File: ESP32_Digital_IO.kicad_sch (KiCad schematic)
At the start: 23 parts, among them J2 217179-0001, J3 DIGITAL_IO_3V3, U3 ESP32-S3-WROOM-1-N16R8

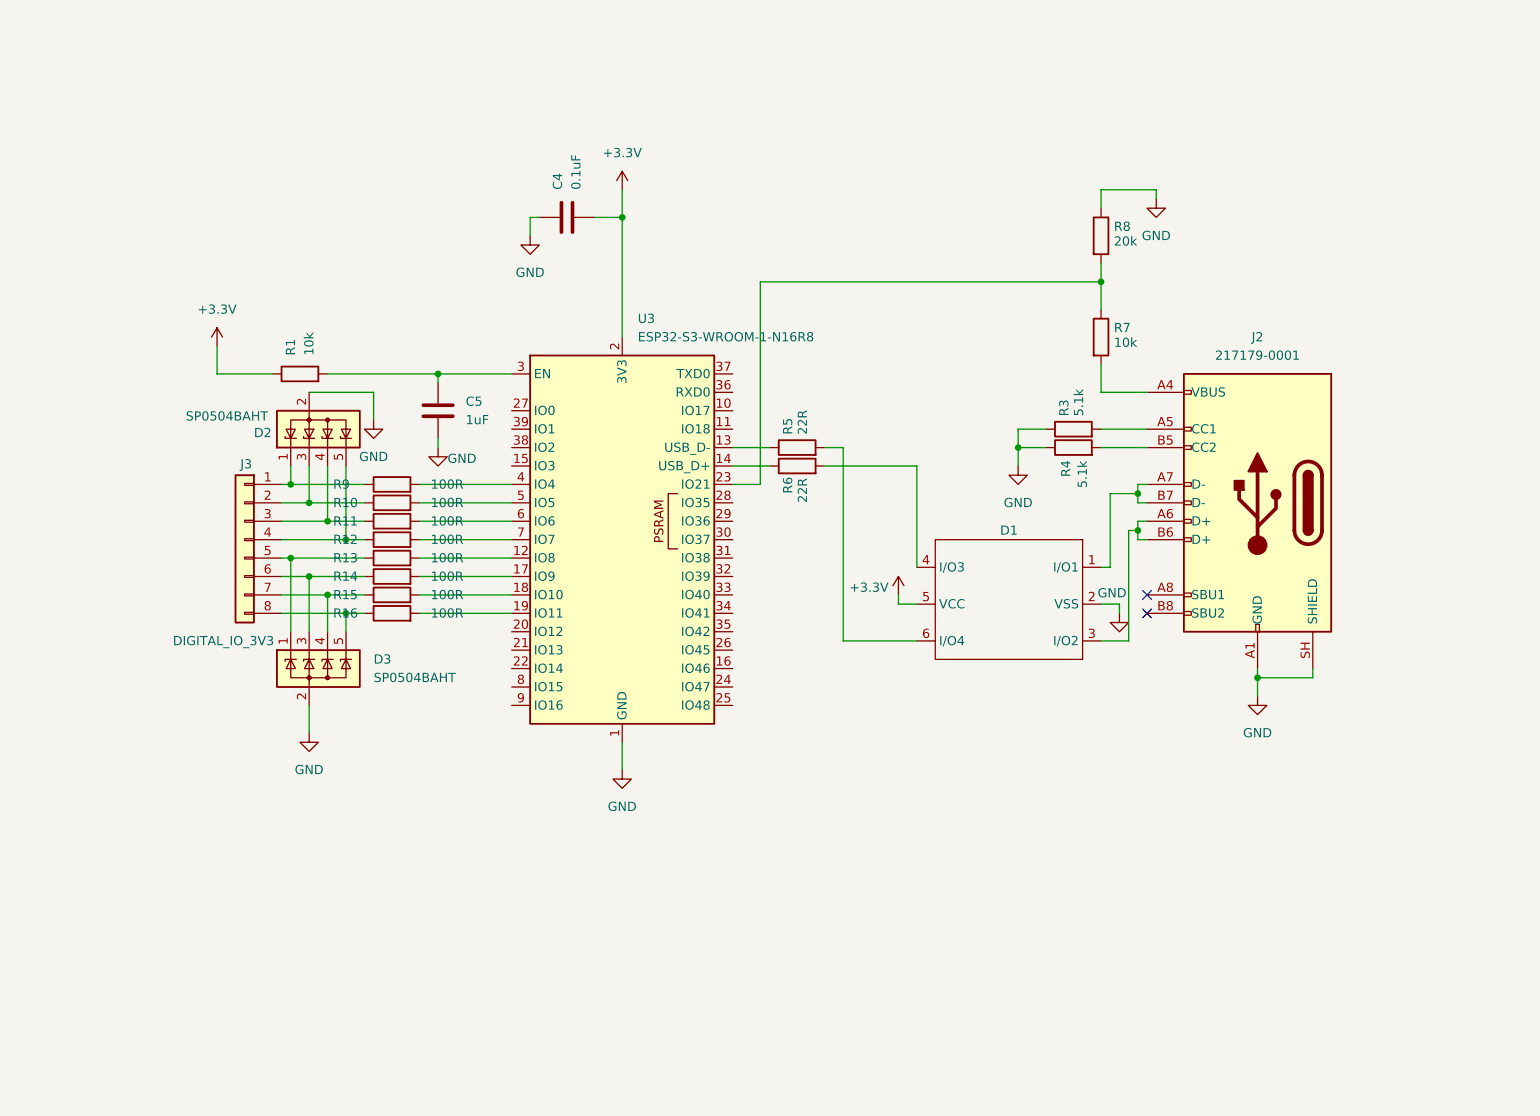
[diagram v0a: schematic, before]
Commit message: added remaining pages. BOM and refinement is all thats left
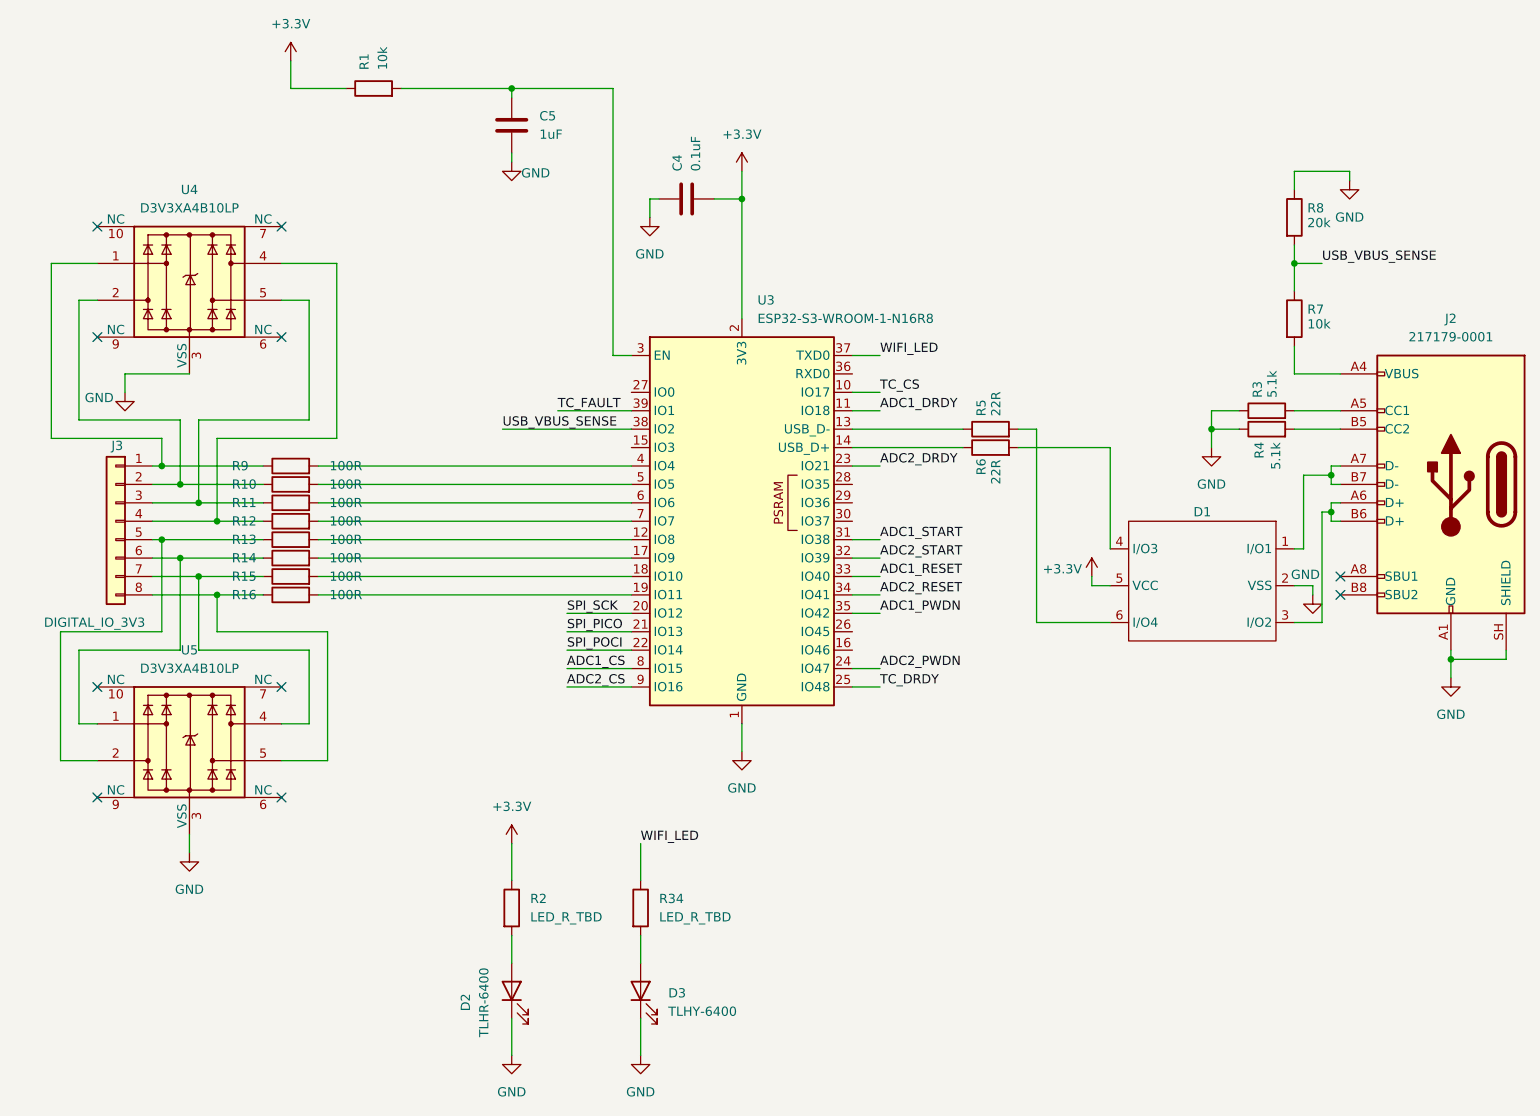
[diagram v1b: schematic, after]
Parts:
- removed D2, D3: SP0504BAHT, Package_TO_SOT_SMD:SOT-23-5, symbol Power_Protection:SP0504BAHT
- added D2: TLHR-6400, LED_SMD:LED_Cree-XHP50_3V_HighDensity, symbol Device:LED
- added D3: TLHY-6400, LED_SMD:LED_Cree-XHP50_3V_HighDensity, symbol Device:LED
- added R2, R34: LED_R_TBD, symbol Device:R
- added U4, U5: D3V3XA4B10LP, Package_DFN_QFN:Diodes_UDFN-10_1x2.5mm_P0.5mm, symbol Power_Protection:D3V3XA4B10LP
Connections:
- net +3.3V: now also R2.1
- net GND: now also D2.1 (K), D3.1 (K), U4.3 (VSS), U4.8 (VSS), U5.3 (VSS), U5.8 (VSS)
- net USB_VBUS_SENSE: now reaches R7.1, R8.2
- net USB_VBUS_SENSE: now also U3.38 (IO2); no longer U3.23 (IO21)
- net at J3.8 (Pin_8), R16.1: now also U5.5
- net at J3.7 (Pin_7), R15.1: now also U5.4
- net at J3.1 (Pin_1), R9.1: now also U4.1
- net at J3.2 (Pin_2), R10.1: now also U4.2
- net at J3.3 (Pin_3), R11.1: now also U4.5
- net at J3.4 (Pin_4), R12.1: now also U4.4
- net at J3.5 (Pin_5), R13.1: now also U5.2
- net at J3.6 (Pin_6), R14.1: now also U5.1
- net TC_CS: now reaches U3.10 (IO17)
- net ADC1_DRDY: now reaches U3.11 (IO18)
- net SPI_SCK: now reaches U3.20 (IO12)
- net SPI_PICO: now reaches U3.21 (IO13)
- net SPI_POCI: now reaches U3.22 (IO14)
- net ADC2_PWDN: now reaches U3.24 (IO47)
- net TC_DRDY: now reaches U3.25 (IO48)
- net ADC1_START: now reaches U3.31 (IO38)
- net ADC2_START: now reaches U3.32 (IO39)
- net ADC1_RESET: now reaches U3.33 (IO40)
- net ADC2_RESET: now reaches U3.34 (IO41)
- net ADC1_PWDN: now reaches U3.35 (IO42)
- net WIFI_LED: now reaches U3.37 (TXD0)
- net WIFI_LED: now also R34.1
- net TC_FAULT: now reaches U3.39 (IO1)
- net ADC1_CS: now reaches U3.8 (IO15)
- net ADC2_CS: now reaches U3.9 (IO16)
- new net: D3.2 (A), R34.2
- new net: D2.2 (A), R2.2
- new net ADC2_DRDY: U3.23 (IO21)
- no-connect marks 2 -> 10
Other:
- moved on the sheet: C4, C5, D1, J2, J3, R1, R10, R11, R12, R13, R14, R15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
